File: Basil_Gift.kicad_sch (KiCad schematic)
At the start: 18 parts, among them J1 Micro_SD_Card, J2 UJC-H-G1-SMT-P6-TR-67, SW1 SW_Push, U1 STM32L051K8Tx, U3 TAS2505TRGERQ1

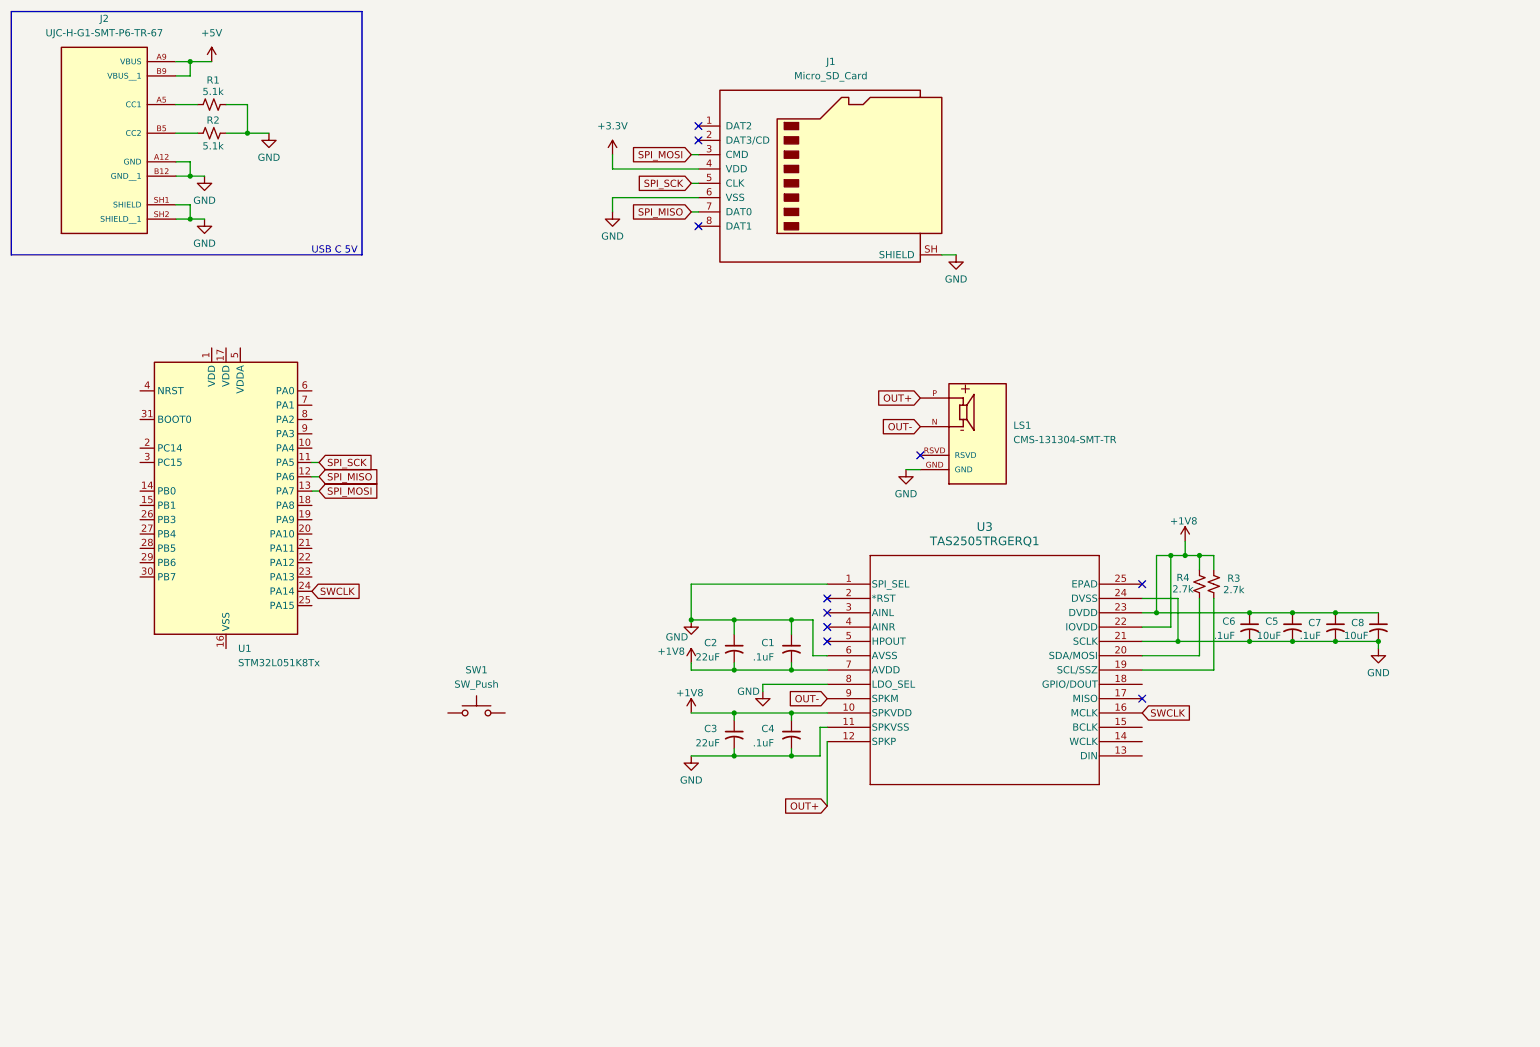
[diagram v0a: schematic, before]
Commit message: schematic done, moving onto fun part
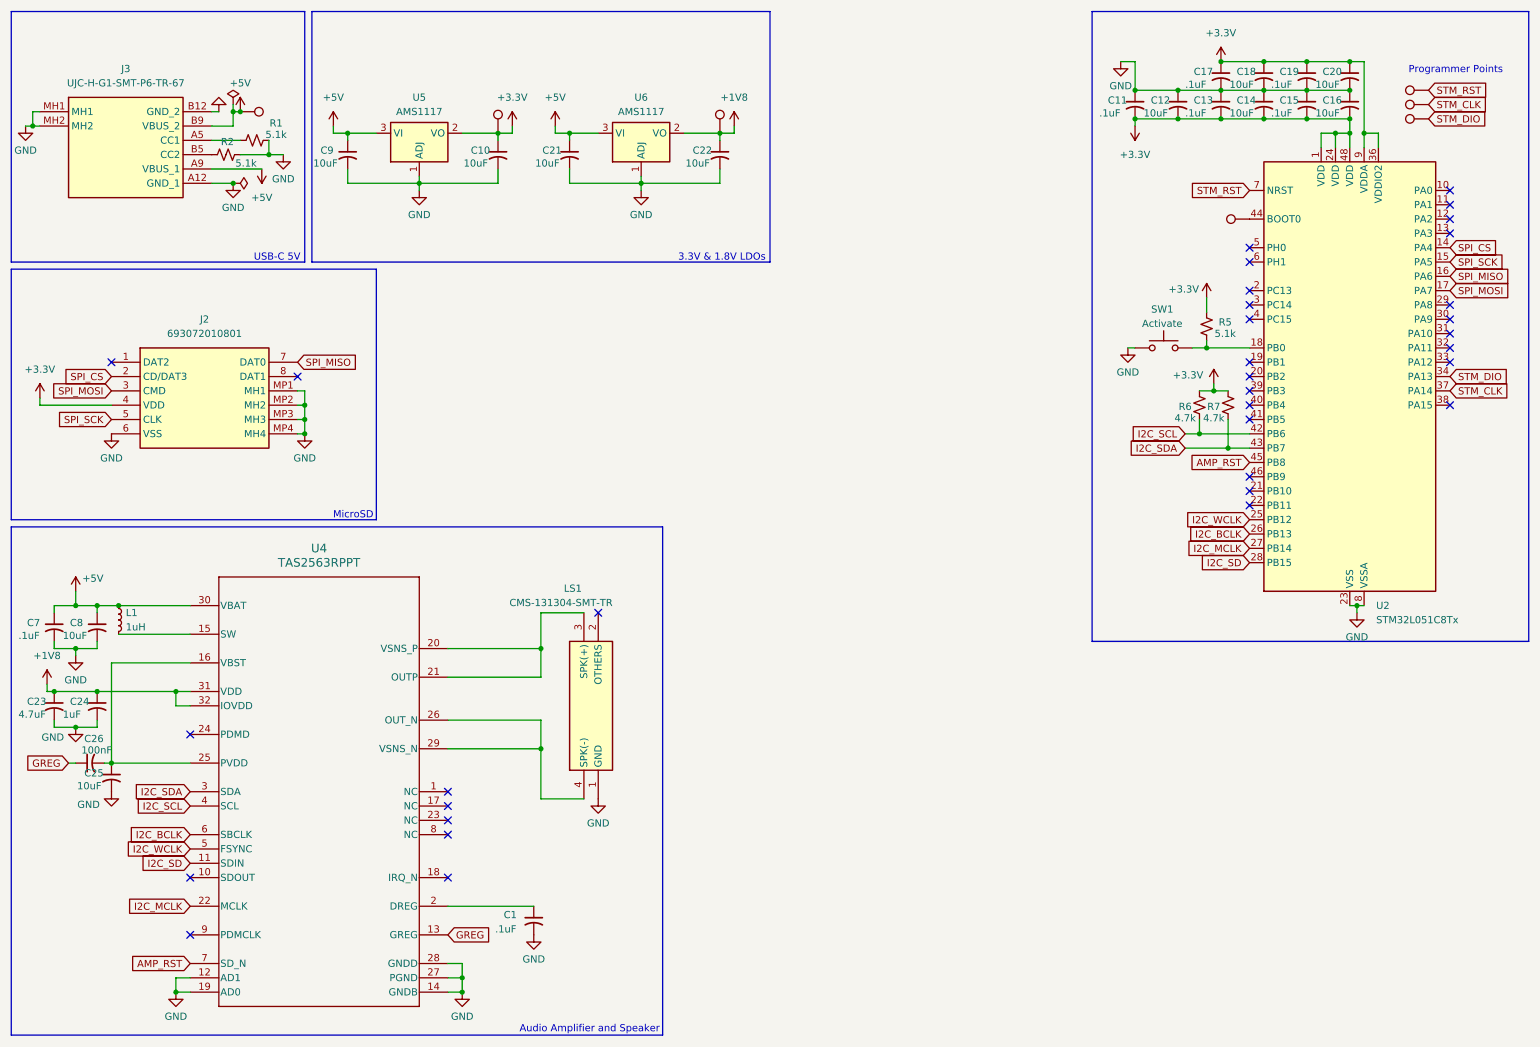
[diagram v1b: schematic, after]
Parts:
- removed C2, C3: 22uF, Capacitor_SMD:C_0603_1608Metric_Pad1.08x0.95mm_HandSolder, symbol Device:C_Small_US
- removed C4, C6: .1uF, Capacitor_SMD:C_0603_1608Metric_Pad1.08x0.95mm_HandSolder, symbol Device:C_Small_US
- removed C5: 10uF, Capacitor_SMD:C_0603_1608Metric_Pad1.08x0.95mm_HandSolder, symbol Device:C_Small_US
- removed J1: Micro_SD_Card, Package_DFN_QFN:TDFN-14-1EP_3x3mm_P0.4mm_EP1.78x2.35mm, symbol Connector:Micro_SD_Card
- removed J2: UJC-H-G1-SMT-P6-TR-67, SamacSys_Parts:SAMESKY_UJC-H-G1-SMT-P6-TR-67, symbol SamacSys_Parts:UJC-H-G1-SMT-P6-TR-67
- removed R3, R4: 2.7k, Resistor_SMD:R_0603_1608Metric_Pad0.98x0.95mm_HandSolder, symbol Device:R_Small_US
- removed U1: STM32L051K8Tx, Package_QFP:LQFP-32_7x7mm_P0.8mm, symbol MCU_ST_STM32L0:STM32L051K8Tx
- removed U3: TAS2505TRGERQ1, SamacSys_Parts:RGE24_2P7X2P7_TEX, symbol SamacSys_Parts:TAS2505TRGERQ1
- added C10, C12, C14, C16, C18, C20, C21, C22, C25, C9: 10uF, Capacitor_SMD:C_0603_1608Metric_Pad1.08x0.95mm_HandSolder, symbol Device:C_Small_US
- added C11, C13, C15, C17, C19: .1uF, Capacitor_SMD:C_0603_1608Metric_Pad1.08x0.95mm_HandSolder, symbol Device:C_Small_US
- added C23: 4.7uF, Capacitor_SMD:C_0603_1608Metric_Pad1.08x0.95mm_HandSolder, symbol Device:C_Small_US
- added C24: 1uF, Capacitor_SMD:C_0603_1608Metric_Pad1.08x0.95mm_HandSolder, symbol Device:C_Small_US
- added C26: 100nF, Capacitor_SMD:C_0603_1608Metric_Pad1.08x0.95mm_HandSolder, symbol Device:C_Small_US
- added J2: 693072010801, Kitty:693072010801, symbol Kitty:693072010801
- added J3: UJC-H-G1-SMT-P6-TR-67, Kitty:UJCHG1SMTP6TR67, symbol Kitty:UJC-H-G1-SMT-P6-TR-67
- added L1: 1uH, Inductor_SMD:L_0603_1608Metric_Pad1.05x0.95mm_HandSolder, symbol Device:L_Small
- added R5: 5.1k, Resistor_SMD:R_0603_1608Metric_Pad0.98x0.95mm_HandSolder, symbol Device:R_Small_US
- added R6, R7: 4.7k, Resistor_SMD:R_0603_1608Metric_Pad0.98x0.95mm_HandSolder, symbol Device:R_Small_US
- added TP1, TP10, TP2, TP4, TP7, TP8, TP9: TestPoint, TestPoint:TestPoint_Pad_D1.5mm, symbol Connector:TestPoint
- added U2: STM32L051C8Tx, Package_QFP:LQFP-48_7x7mm_P0.5mm, symbol MCU_ST_STM32L0:STM32L051C8Tx
- added U4: TAS2563RPPT, Kitty:RPP0032B-MFG, symbol Kitty:TAS2563RPPT
- added U5, U6: AMS1117, Package_TO_SOT_SMD:SOT-223-3_TabPin2, symbol Regulator_Linear:AMS1117
- LS1: footprint SamacSys_Parts:SPKR_CMS-131304-SMT-TR -> Kitty:CMS131304SMTTR; symbol SamacSys_Parts:CMS-131304-SMT-TR -> Kitty:CMS-131304-SMT-TR; Height (none) -> 4.2; Manufacturer_Name (none) -> Same Sky; Manufacturer_Part_Number (none) -> CMS-131304-SMT-TR; Mouser Part Number (none) -> 179-CMS-131304-SMTTR; Mouser Price/Stock (none) -> https://www.mouser.co.uk/ProductDetail/Same-Sky/CMS-131304-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
- SW1: value SW_Push -> Activate; footprint (none) -> Button_Switch_SMD:SW_SPST_EVQP0
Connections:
- net +1V8: now also C22.1, C23.1, C24.1, TP10.1, U4.31 (VDD), U4.32 (IOVDD), U6.2 (VO); no longer C1.2, C7.1, C8.1
- net +3.3V: now also C10.1, C11.2, C12.2, C13.2, C14.2, C15.2, C16.2, C17.1, C18.1, C19.1, C20.1, J2.4 (VDD), R5.2, R6.2, R7.2, TP4.1, U2.1 (VDD), U2.24 (VDD), U2.36 (VDDIO2), U2.48 (VDD), U2.9 (VDDA), U5.2 (VO)
- net +5V: now also C7.1, C8.1, C21.1, C9.1, J3.A9 (VBUS_1), J3.B9 (VBUS_2), L1.1, TP2.1, U4.30 (VBAT), U5.3 (VI), U6.3 (VI)
- net GND: now also C1.2, LS1.1 (GND), SW1.1, C10.2, C11.1, C12.1, C13.1, C14.1, C15.1, C16.1, C17.2, C18.2, C19.2, C20.2, C21.2, C22.2, C23.2, C24.2, C25.2, C9.2, J2.6 (VSS), J2.MP1 (MH1), J2.MP2 (MH2), J2.MP3 (MH3), J2.MP4 (MH4), J3.A12 (GND_1), J3.B12 (GND_2), J3.MH1, J3.MH2, U2.23 (VSS), U2.35 (VSS), U2.47 (VSS), U2.8 (VSSA), U4.12 (AD1), U4.14 (GNDB), U4.19 (AD0), U4.27 (PGND), U4.28 (GNDD), U5.1 (ADJ), U6.1 (ADJ); no longer C1.1, LS1.GND
- net SPI_MISO: now also J2.7 (DAT0), U2.16 (PA6)
- net SPI_MOSI: now also J2.3 (CMD), U2.17 (PA7)
- net SPI_SCK: now also J2.5 (CLK), U2.15 (PA5)
- net at R2.1: now also J3.B5 (CC2)
- net at R1.1: now also J3.A5 (CC1)
- net at SW1.2: now also R5.1, U2.18 (PB0)
- removed net OUT+: LS1.P
- removed net OUT-: LS1.N
- new net: TP1.1, U2.44 (BOOT0)
- new net: C25.1, C26.2, U4.16 (VBST), U4.25 (PVDD)
- new net: L1.2, U4.15 (SW)
- new net: C1.1, U4.2 (DREG)
- new net: LS1.3 (SPK(+)), U4.20 (VSNS_P), U4.21 (OUTP)
- new net: LS1.4 (SPK(-)), U4.26 (OUT_N), U4.29 (VSNS_N)
- new net AMP_RST: U2.45 (PB8), U4.7 (SD_N)
- new net GREG: C26.1, U4.13 (GREG)
- new net I2C_BCLK: U2.26 (PB13), U4.6 (SBCLK)
- new net I2C_MCLK: U2.27 (PB14), U4.22 (MCLK)
- new net I2C_SCL: R6.1, U2.42 (PB6), U4.4 (SCL)
- new net I2C_SD: U2.28 (PB15), U4.11 (SDIN)
- new net I2C_SDA: R7.1, U2.43 (PB7), U4.3 (SDA)
- new net I2C_WCLK: U2.25 (PB12), U4.5 (FSYNC)
- new net SPI_CS: J2.2 (CD/DAT3), U2.14 (PA4)
- new net STM_CLK: TP8.1, U2.37 (PA14)
- new net STM_DIO: TP9.1, U2.34 (PA13)
- new net STM_RST: TP7.1, U2.7 (NRST)
- no-connect marks 10 -> 34
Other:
- note added: "3.3V & 1.8V LDOs"
- note added: "Audio Amplifier and Speaker"
- note added: "MicroSD"
- note added: "Programmer Points"
- note added: "USB-C 5V"
- note removed: "USB C 5V"
- moved on the sheet: SW1
